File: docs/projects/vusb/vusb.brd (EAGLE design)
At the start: 48.2 x 27.6 mm, 16 parts

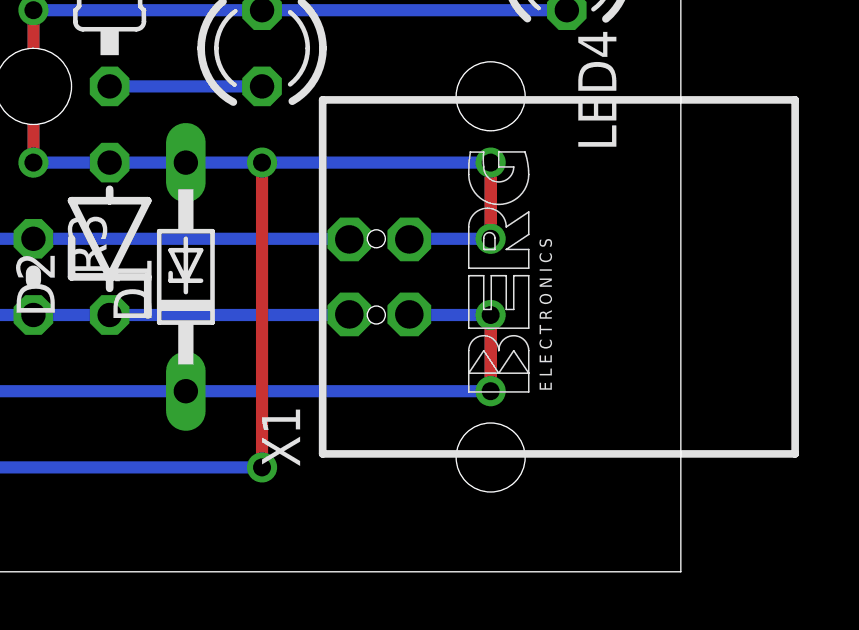
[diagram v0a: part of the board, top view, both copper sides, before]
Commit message: fix airwires
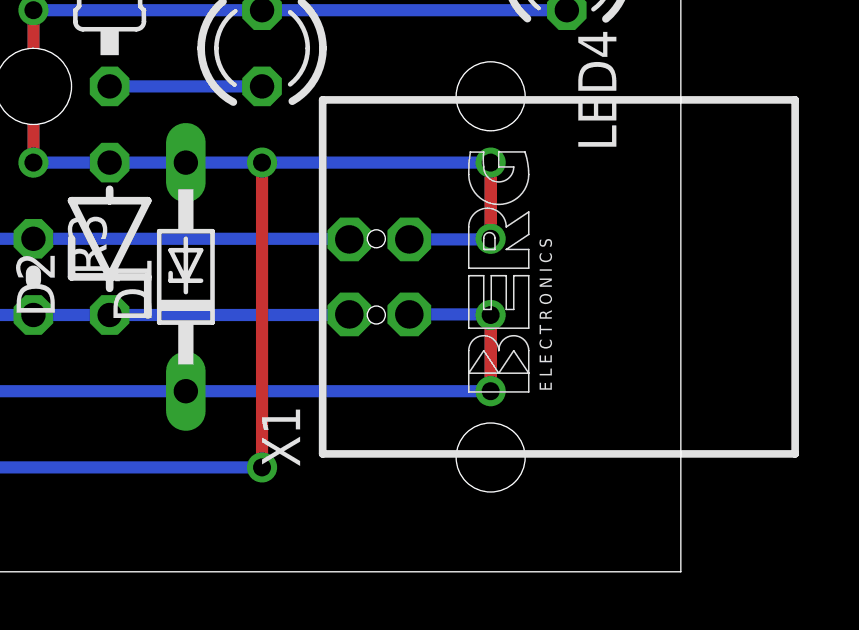
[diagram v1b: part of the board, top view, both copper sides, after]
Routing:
- net GND: track 94.2 -> 96.7 mm, vias 4 -> 6
- net N$18: track 2.54 -> 0.00 mm, vias 2 -> 0
- net N$19: track 2.54 -> 0.00 mm, vias 2 -> 0
- net N$2: track 23.1 -> 25.6 mm, vias 0 -> 2
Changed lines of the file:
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@@
 <contactref element="R2" pad="1"/>
 <contactref element="D1" pad="C"/>
+<wire x1="33.02" y1="7.62" x2="43.18" y2="7.62" width="0.4064" layer="16"/>
 <wire x1="43.18" y1="7.62" x2="53.34" y2="7.62" width="0.4064" layer="16"/>
-<wire x1="50.63" y1="10.18" x2="50.63" y2="10.16" width="0.4064" layer="16"/>
-<wire x1="50.63" y1="10.16" x2="53.34" y2="10.16" width="0.4064" layer="16"/>
-<wire x1="33.02" y1="7.62" x2="43.18" y2="7.62" width="0.4064" layer="16"/>
-<wire x1="53.34" y1="7.62" x2="53.34" y2="10.16" width="0" layer="19" extent="16-16"/>
+<via x="53.34" y="10.16" extent="1-16" drill="0.6" shape="square"/>
+<via x="53.34" y="7.62" extent="1-16" drill="0.6" shape="square"/>
+<wire x1="53.34" y1="7.62" x2="53.34" y2="10.16" width="0.4064" layer="1"/>
+<wire x1="50.63" y1="10.18" x2="53.34" y2="10.18" width="0.4064" layer="16"/>
+<wire x1="53.34" y1="10.18" x2="53.34" y2="10.16" width="0.4064" layer="16"/>
 </signal>
 <signal name="N$3">
@@
 <wire x1="12.7" y1="27.94" x2="17.78" y2="27.94" width="0.4064" layer="16"/>
 </signal>
-<signal name="N$18">
-<wire x1="53.34" y1="15.24" x2="53.34" y2="12.7" width="0.4064" layer="1"/>
-<via x="53.34" y="12.7" extent="1-16" drill="0.6" shape="square"/>
-<via x="53.34" y="15.24" extent="1-16" drill="0.6" shape="square"/>
-</signal>
-<signal name="N$19">
-<wire x1="53.34" y1="10.16" x2="53.34" y2="7.62" width="0.4064" layer="1"/>
-<via x="53.34" y="10.16" extent="1-16" drill="0.6" shape="square"/>
-<via x="53.34" y="7.62" extent="1-16" drill="0.6" shape="square"/>
-</signal>
 <signal name="N$7">
 <contactref element="R1" pad="2"/>
@@
 <contactref element="C2" pad="-"/>
 <contactref element="C1" pad="2"/>
-<wire x1="45.72" y1="15.24" x2="53.34" y2="15.24" width="0.4064" layer="16"/>
 <wire x1="12.7" y1="5.08" x2="27.94" y2="5.08" width="0.4064" layer="16"/>
 <wire x1="27.94" y1="5.08" x2="22.86" y2="5.08" width="0.4064" layer="16"/>
 <wire x1="22.86" y1="5.08" x2="45.72" y2="5.08" width="0.4064" layer="16"/>
 <wire x1="45.72" y1="5.08" x2="45.72" y2="15.24" width="0.4064" layer="1"/>
-<wire x1="50.63" y1="12.68" x2="50.63" y2="12.7" width="0.4064" layer="16"/>
-<wire x1="50.63" y1="12.7" x2="53.34" y2="12.7" width="0.4064" layer="16"/>
 <wire x1="43.18" y1="15.24" x2="40.64" y2="15.24" width="0.4064" layer="16"/>
 <wire x1="45.72" y1="15.24" x2="43.18" y2="15.24" width="0.4064" layer="16"/>
@@
 <wire x1="45.72" y1="20.32" x2="55.88" y2="20.32" width="0.4064" layer="16"/>
 <wire x1="38.1" y1="15.24" x2="38.1" y2="20.32" width="0.4064" layer="1"/>
-<wire x1="53.34" y1="15.24" x2="53.34" y2="12.7" width="0" layer="19" extent="16-16"/>
 <via x="45.72" y="5.08" extent="1-16" drill="0.6" shape="square"/>
 <via x="45.72" y="15.24" extent="1-16" drill="0.6" shape="square"/>
 <via x="38.1" y="15.24" extent="1-16" drill="0.6" shape="square"/>
 <via x="38.1" y="20.32" extent="1-16" drill="0.6" shape="square"/>
+<wire x1="45.72" y1="15.24" x2="53.34" y2="15.24" width="0.4064" layer="16"/>
+<wire x1="50.63" y1="12.68" x2="53.34" y2="12.68" width="0.4064" layer="16"/>
+<wire x1="53.34" y1="12.68" x2="53.34" y2="12.7" width="0.4064" layer="16"/>
+<via x="53.34" y="12.7" extent="1-16" drill="0.6" shape="square"/>
+<via x="53.34" y="15.24" extent="1-16" drill="0.6" shape="square"/>
+<wire x1="53.34" y1="15.24" x2="53.34" y2="12.7" width="0.4064" layer="1"/>
 </signal>
 </signals>
